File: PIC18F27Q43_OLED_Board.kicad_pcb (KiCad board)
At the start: 2 copper layers, 55 parts, among them J1 Conn_PIC_ICSP_ICD, J2 OLED_Connector, J4 USB_B_Mini, Q1 C143946, SW1 SW_Push, SW2 SW_Push, SW3 SW_Push, SW4 SW_Push, SW5 SW_SPDT, U1 PIC18F27Q43-I/STX, U2 C51118

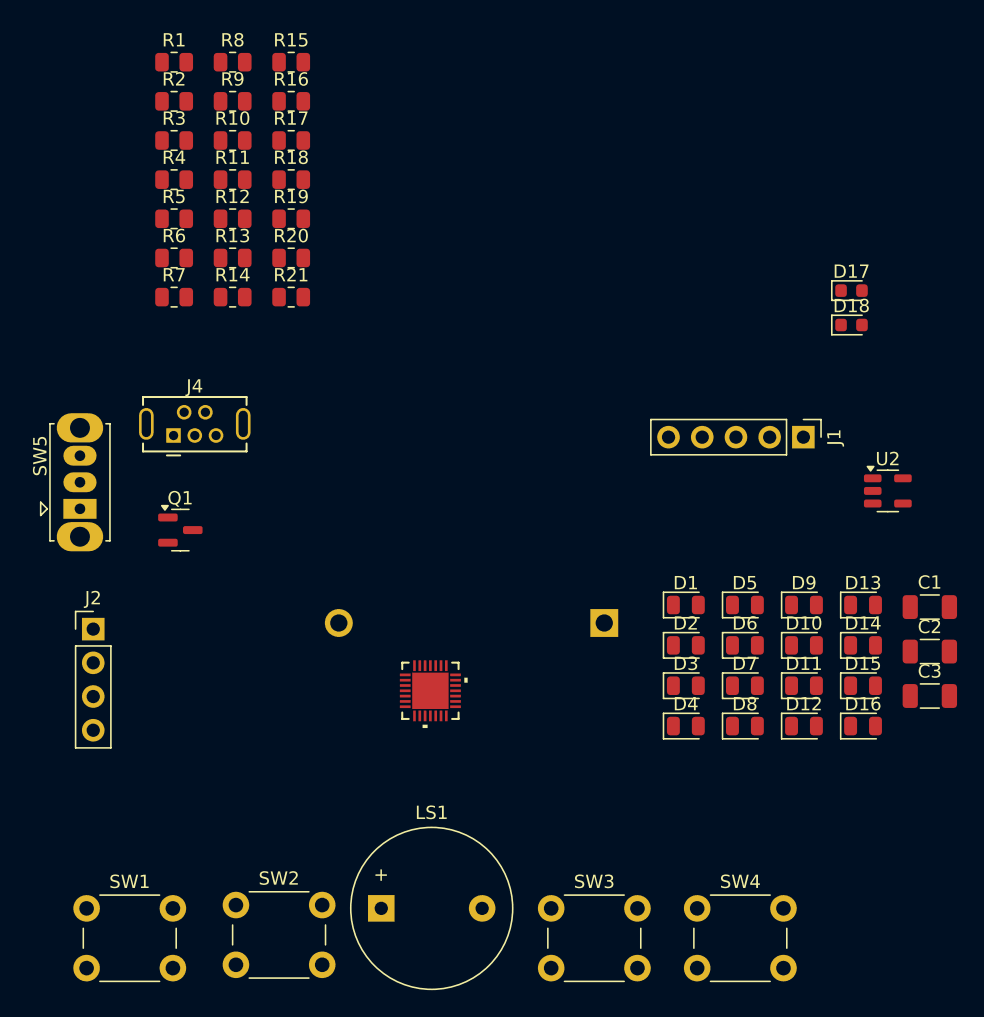
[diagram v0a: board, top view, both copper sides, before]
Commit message: Rev.1 : PCB Design finished.
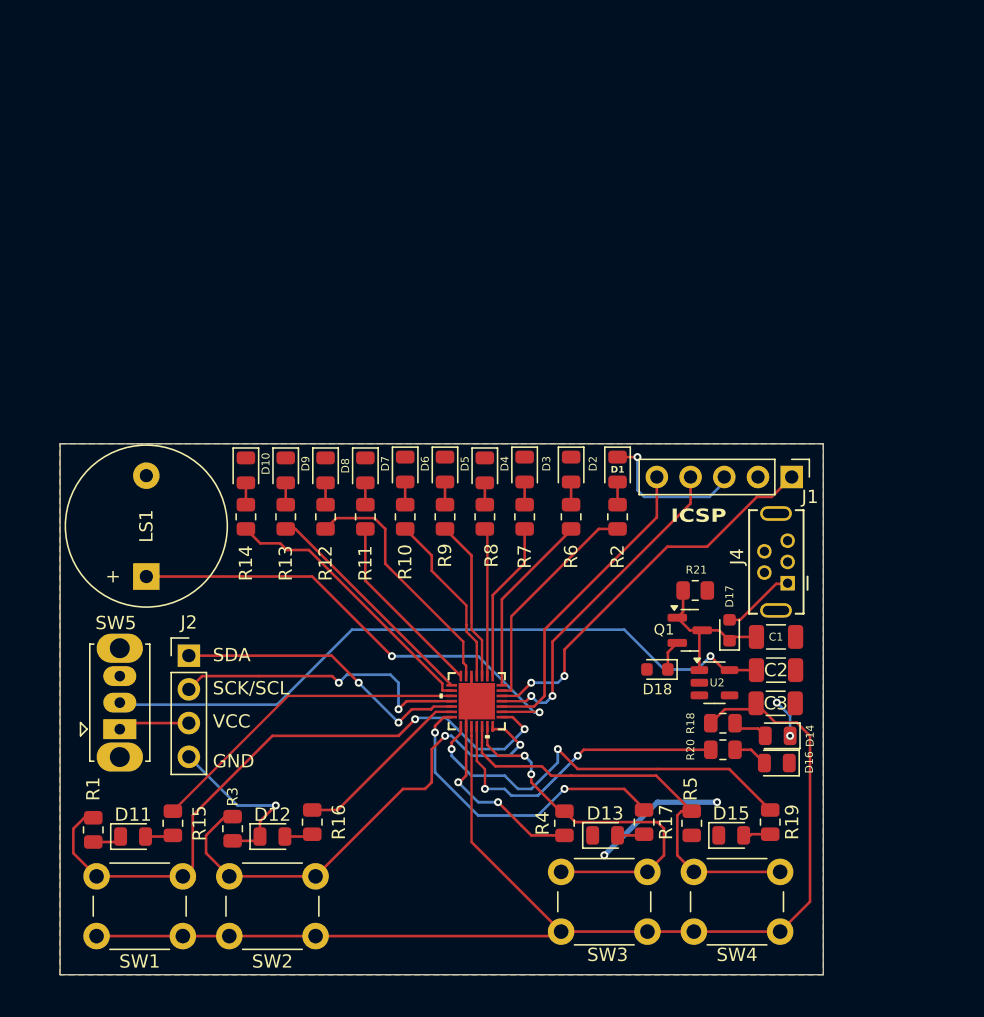
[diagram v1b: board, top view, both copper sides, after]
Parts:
- removed BT1: V, Battery:BatteryHolder_ComfortableElectronic_CH273-2450_1x2450
- moved R5 60.0 mm to (139.6, 111.1), turned to 90 degrees
- moved R1 58.2 mm to (94.5, 111.6), turned to 90 degrees
- moved R19 58.0 mm to (145.5, 111.0), turned to -90 degrees
- moved R15 58.0 mm to (100.5, 111.1), turned to -90 degrees
- moved R17 57.8 mm to (136.0, 111.0), turned to -90 degrees
- moved R4 56.7 mm to (130.0, 111.1), turned to 90 degrees
- moved R16 54.3 mm to (111.0, 111.0), turned to -90 degrees
- moved R18 52.3 mm to (141.9, 103.5)
- moved R3 52.0 mm to (105.0, 111.5), turned to 90 degrees
- moved D11 51.8 mm to (97.5, 112.1)
- moved R20 49.3 mm to (141.9, 105.5)
- moved J4 47.6 mm to (146.8, 93.0), turned to 90 degrees
- moved R2 45.8 mm to (134.0, 88.0), turned to 90 degrees
- moved D10 44.1 mm to (106.0, 84.5), turned to -90 degrees
- moved D12 40.9 mm to (108.0, 112.1)
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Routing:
- net VCC: track 0.00 -> 100.1 mm
- net GND: track 0.00 -> 59.1 mm, vias 0 -> 8
- net Net-(SW5-B): track 0.00 -> 52.5 mm, vias 0 -> 1
- net /RB4: track 0.00 -> 49.3 mm, vias 0 -> 2
- net /RB3: track 0.00 -> 38.0 mm, vias 0 -> 2
- net /RB5: track 0.00 -> 36.7 mm, vias 0 -> 2
- net /RB1: track 0.00 -> 32.1 mm
- net /RC7: track 0.00 -> 31.3 mm, vias 0 -> 2
- net /MCLR: track 0.00 -> 30.5 mm, vias 0 -> 2
- net /RB2: track 0.00 -> 28.5 mm, vias 0 -> 2
- net /PGD: track 0.00 -> 25.3 mm, vias 0 -> 2
- net /RC2: track 0.00 -> 24.6 mm
- net /PGC: track 0.00 -> 23.7 mm
- net /RC6: track 0.00 -> 23.7 mm, vias 0 -> 2
- net /RB0: track 0.00 -> 23.6 mm, vias 0 -> 2
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- added copper zone on F.Cu, net GND
- added copper zone on B.Cu, net VCC
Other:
- board outline added: 57.5 x 40 mm
- board text added: "GND"
- board text added: "ICSP"
- board text added: "KiCAD"
- board text added: "Made with"
- board text added: "OLED Board PIC18F27Q43 Rev.1: 28th March 2025 Designed by @deulamco"
- board text added: "SCK/SCL"
- board text added: "SDA"
- board text added: "VCC"
